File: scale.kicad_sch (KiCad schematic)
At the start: 10 parts, among them J1 Conn_01x02_Pin, J2 Conn_01x04_Pin, J4 Conn_01x05_Pin

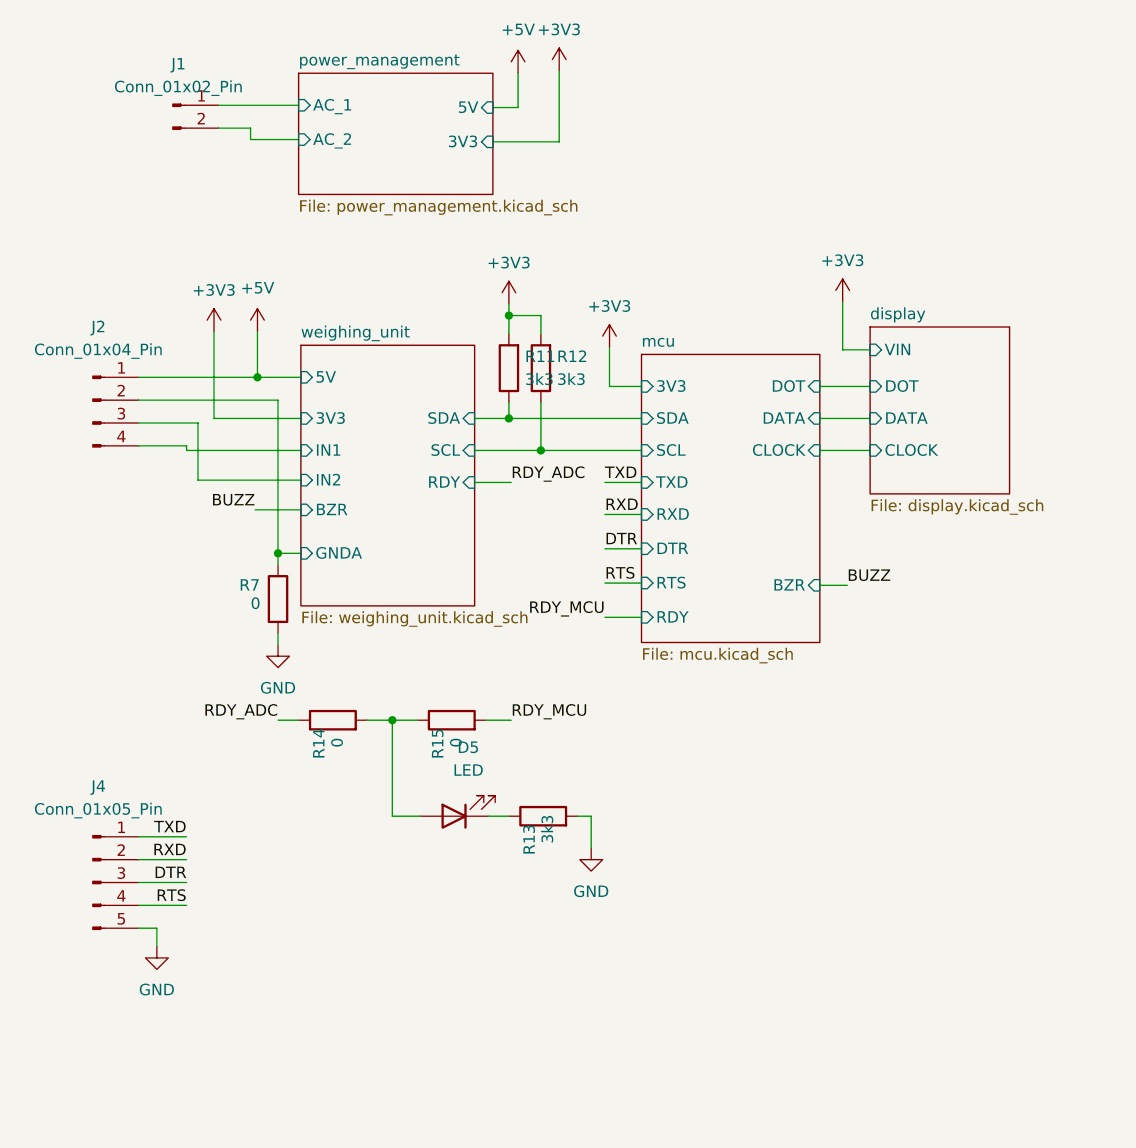
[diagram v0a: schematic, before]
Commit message: start routing
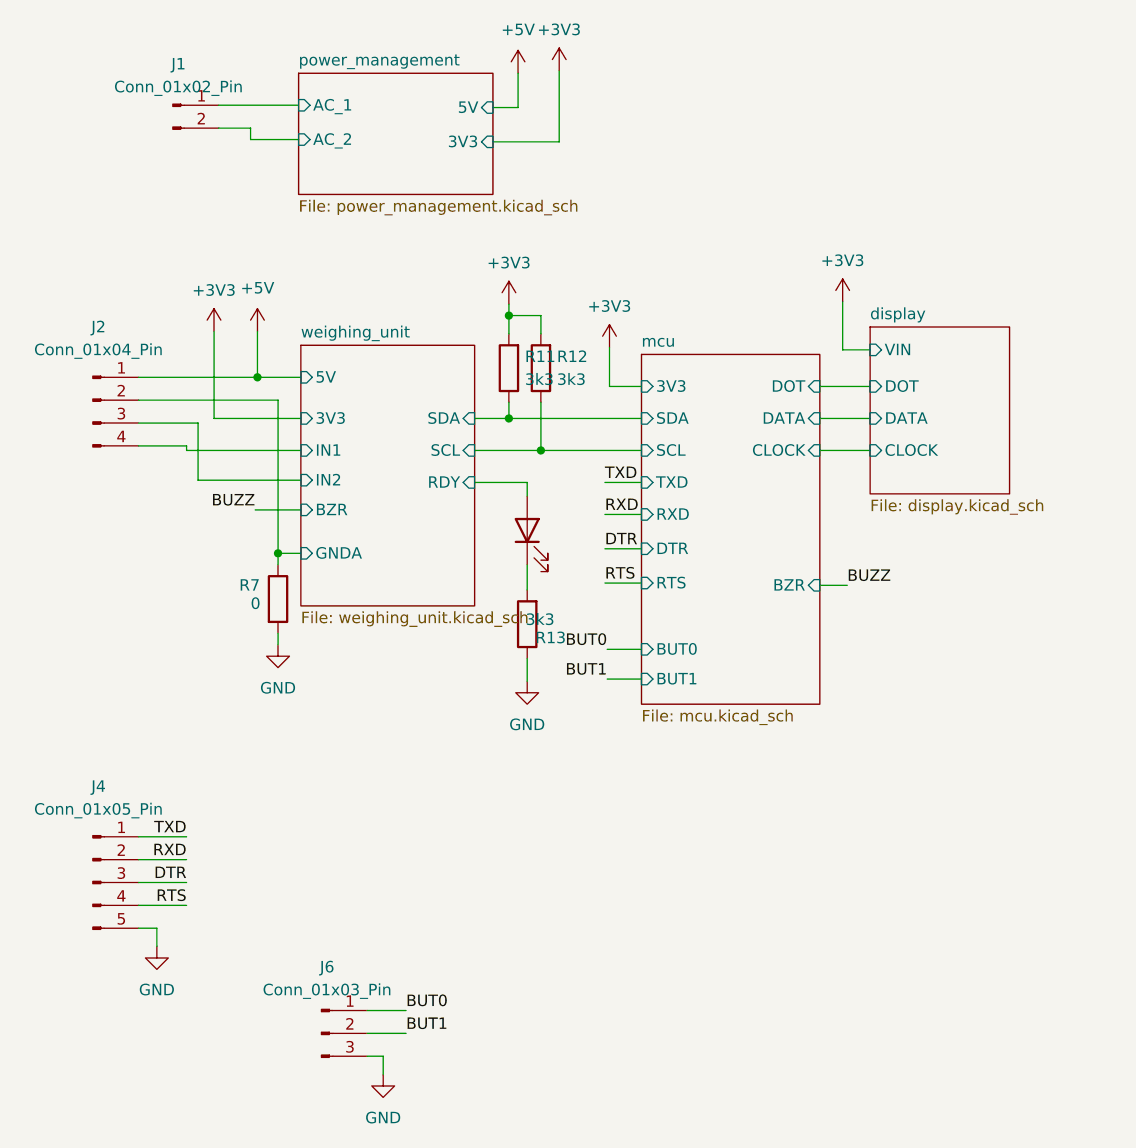
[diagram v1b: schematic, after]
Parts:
- removed R14, R15: 0, Resistor_SMD:R_0402_1005Metric, symbol Device:R
- added J6: Conn_01x03_Pin, BBG:CONN_S3B-XH-ALFSN_JST, symbol Connector:Conn_01x03_Pin
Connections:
- net GND: now also R13.1, J6.3 (Pin_3); no longer R13.2
- net weighing_unit/RDY: now reaches D5.2 (A)
- net at D5.1 (K): now also R13.2; no longer R13.1
- new net BUT0: J6.1 (Pin_1)
- new net BUT1: J6.2 (Pin_2)
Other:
- sheet mcu ports: added BUT0, BUT1; removed RDY
- moved on the sheet: R13
